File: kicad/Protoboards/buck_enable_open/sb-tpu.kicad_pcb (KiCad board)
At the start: 6 copper layers, 128 x 116 mm, 19 parts, among them IC1 LM3370SD-4221/NOPB, U1 LTC4413EDD-1_TRPBF

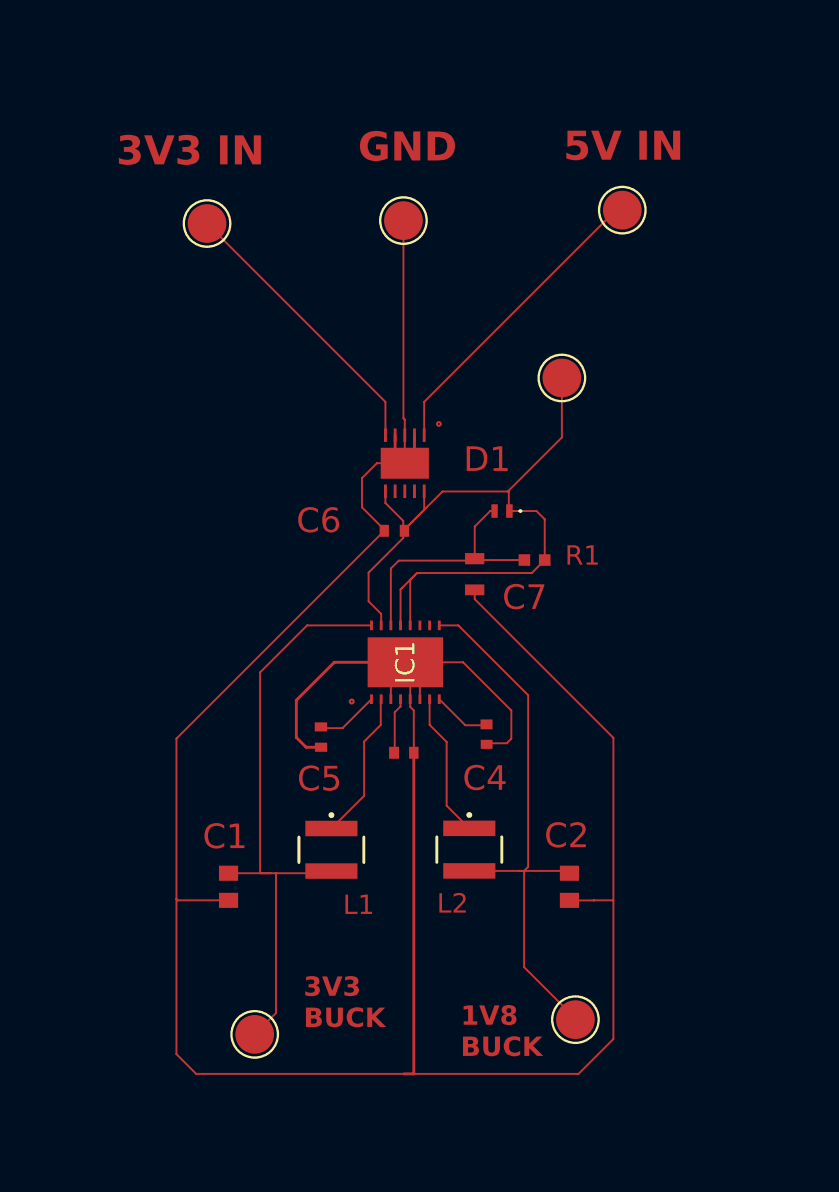
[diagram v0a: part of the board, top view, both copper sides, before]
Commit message: [proto] Dead bug gambit
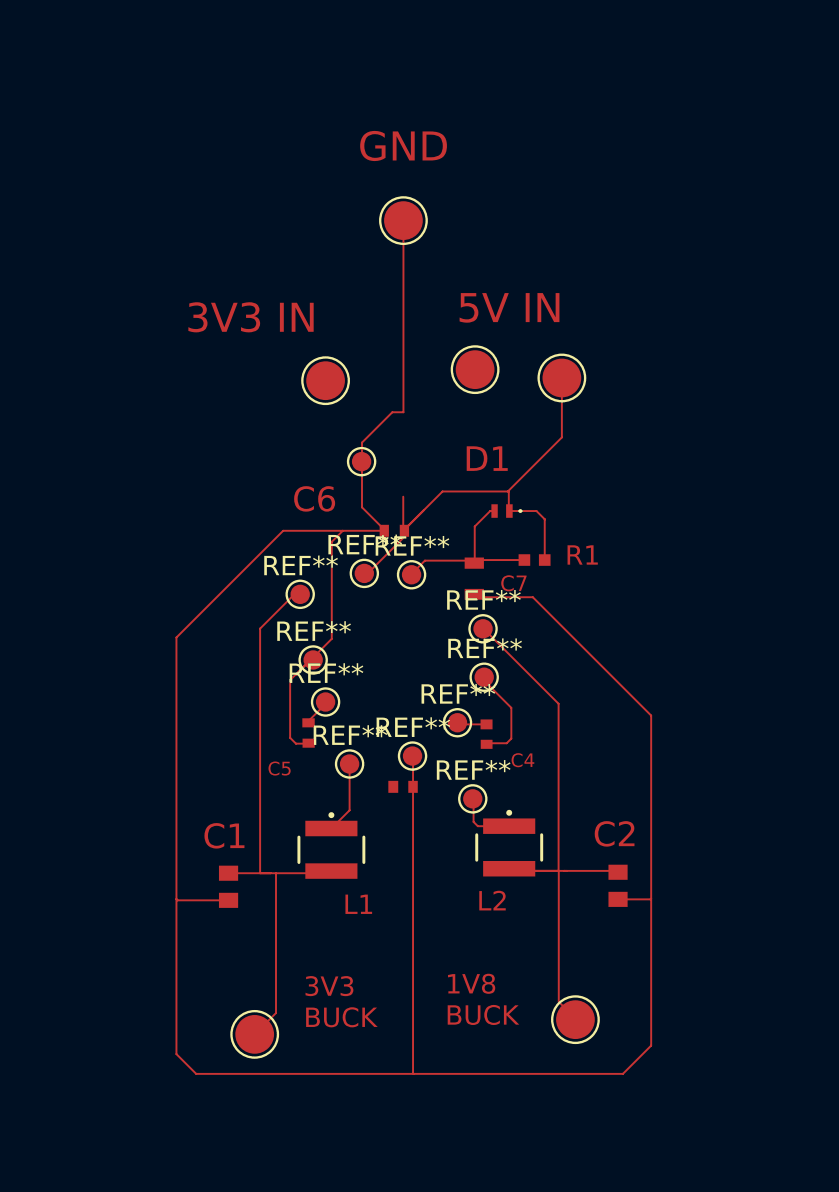
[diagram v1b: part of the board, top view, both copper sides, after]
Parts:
- removed IC1: LM3370SD-4221/NOPB, footprints:SDA16B
- removed U1: LTC4413EDD-1_TRPBF, footprints:DFN-10_DD
- added REF**: TestPoint_Pad_D1.0mm, TestPoint:TestPoint_Pad_D1.0mm, F.Cu at (137.2, 92.7)
- added REF**: TestPoint_Pad_D1.0mm, TestPoint:TestPoint_Pad_D1.0mm, F.Cu at (135.3, 105.1)
- added REF**: TestPoint_Pad_D1.0mm, TestPoint:TestPoint_Pad_D1.0mm, F.Cu at (134.0, 99.6)
- added REF**: TestPoint_Pad_D1.0mm, TestPoint:TestPoint_Pad_D1.0mm, F.Cu at (137.3, 98.5)
- added REF**: TestPoint_Pad_D1.0mm, TestPoint:TestPoint_Pad_D1.0mm, F.Cu at (142.1, 106.2)
- added REF**: TestPoint_Pad_D1.0mm, TestPoint:TestPoint_Pad_D1.0mm, F.Cu at (136.6, 108.3)
- added REF**: TestPoint_Pad_D1.0mm, TestPoint:TestPoint_Pad_D1.0mm, F.Cu at (139.8, 98.6)
- added REF**: TestPoint_Pad_D1.0mm, TestPoint:TestPoint_Pad_D1.0mm, F.Cu at (134.7, 103.0)
- added REF**: TestPoint_Pad_D1.0mm, TestPoint:TestPoint_Pad_D1.0mm, F.Cu at (139.8, 107.9)
- added REF**: TestPoint_Pad_D1.0mm, TestPoint:TestPoint_Pad_D1.0mm, F.Cu at (143.5, 103.9)
- added REF**: TestPoint_Pad_D1.0mm, TestPoint:TestPoint_Pad_D1.0mm, F.Cu at (142.9, 110.1)
- added REF**: TestPoint_Pad_D1.0mm, TestPoint:TestPoint_Pad_D1.0mm, F.Cu at (143.4, 101.4)
- moved TP3 11.2 mm to (143.0, 88.0)
- moved TP4 10.2 mm to (135.3, 88.5)
- moved C2 2.51 mm to (150.4, 114.6)
- moved L2 2.06 mm to (144.8, 112.7)
- moved C3 1.76 mm to (139.3, 109.5)
- moved C5 0.67 mm to (134.4, 106.7)
- moved C7 0.23 mm to (143.0, 98.8)
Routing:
- net VSYS: track 51.3 -> 27.1 mm
- net VSYS_DA: track 16.1 -> 0.00 mm
- net +3V3: track 14.7 -> 0.00 mm
- net GND: track 153.7 -> 146.6 mm
- net Net-(IC1-SW1): track 7.52 -> 2.78 mm
- net Net-(D1-A): track 13.2 -> 8.88 mm
- net Net-(IC1-SW2): track 7.74 -> 4.13 mm
- net VDD_1V8: track 29.0 -> 31.2 mm
- net /BUCK2: track 31.9 -> 30.1 mm
